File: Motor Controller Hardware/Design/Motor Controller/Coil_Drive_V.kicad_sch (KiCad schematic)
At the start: 15 parts, among them Q7 NMOS, Q8 NMOS, U10 AD8418

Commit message: a:
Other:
- title: (none) -> HyperDrive Motor Controller
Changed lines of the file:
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@@
 	(paper "A4")
 	(title_block
-		(rev "1")
+		(title "HyperDrive Motor Controller")
+		(rev "Mk. 1")
 		(company "University of Alberta EcoCar Team")
 	)

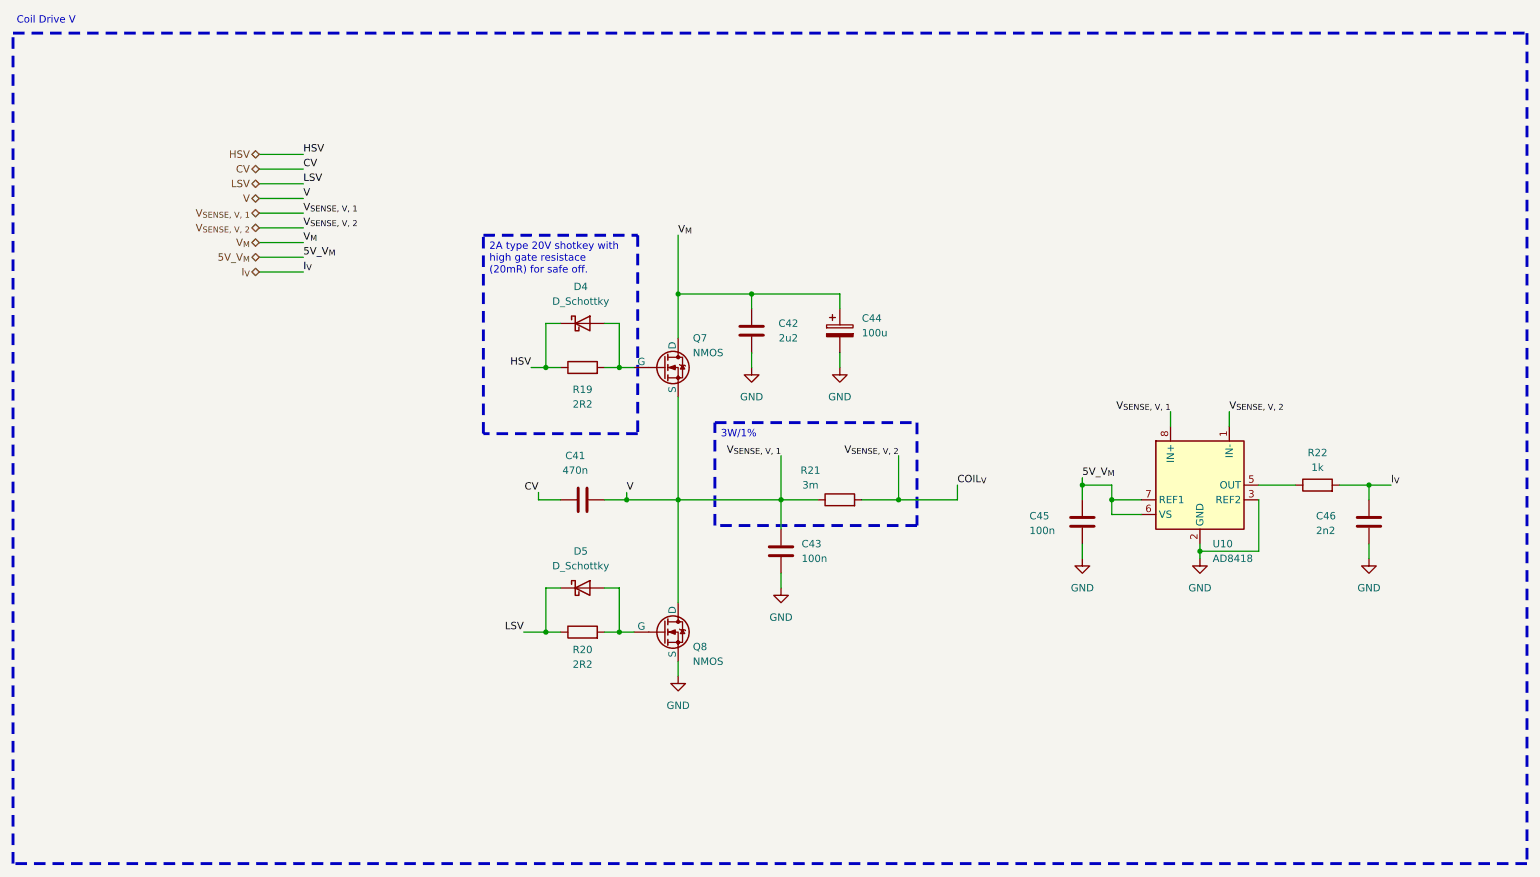
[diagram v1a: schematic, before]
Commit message: A
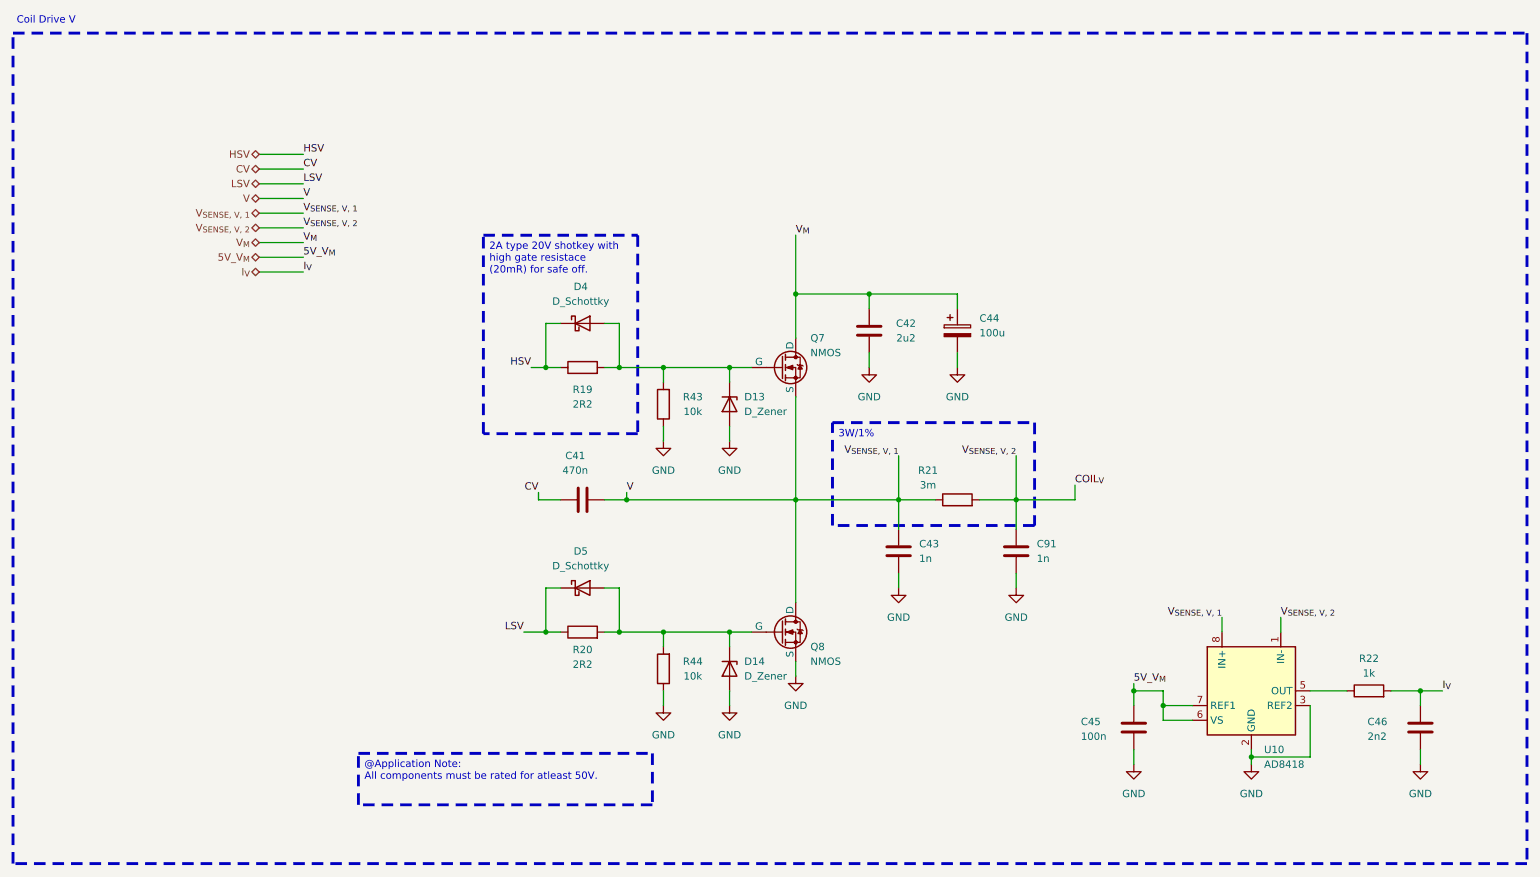
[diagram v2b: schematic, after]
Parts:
- added C91: 1n, symbol Device:C
- added D13, D14: D_Zener, symbol Device:D_Zener
- added R43, R44: 10k, symbol Device:R
- C43: value 100n -> 1n
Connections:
- net GND: now also C91.2, D13.2 (A), D14.2 (A), R43.1, R44.1
- net V_{SENSE, V, 2}: now also C91.1
- net at D5.2 (A), Q8.2 (G), R20.2: now also D14.1 (K), R44.2
- net at D4.2 (A), Q7.2 (G), R19.2: now also D13.1 (K), R43.2
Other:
- moved on the sheet: C42, C43, C44, C45, C46, Q7, Q8, R21, R22, U10
